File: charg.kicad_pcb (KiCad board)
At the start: 2 copper layers, 13 parts, among them IC1 SI3483DDV-T1-BE3, IC2 BQ25302RTER, J1 Screw_Terminal_01x04, J2 Screw_Terminal_01x04, J4 EN

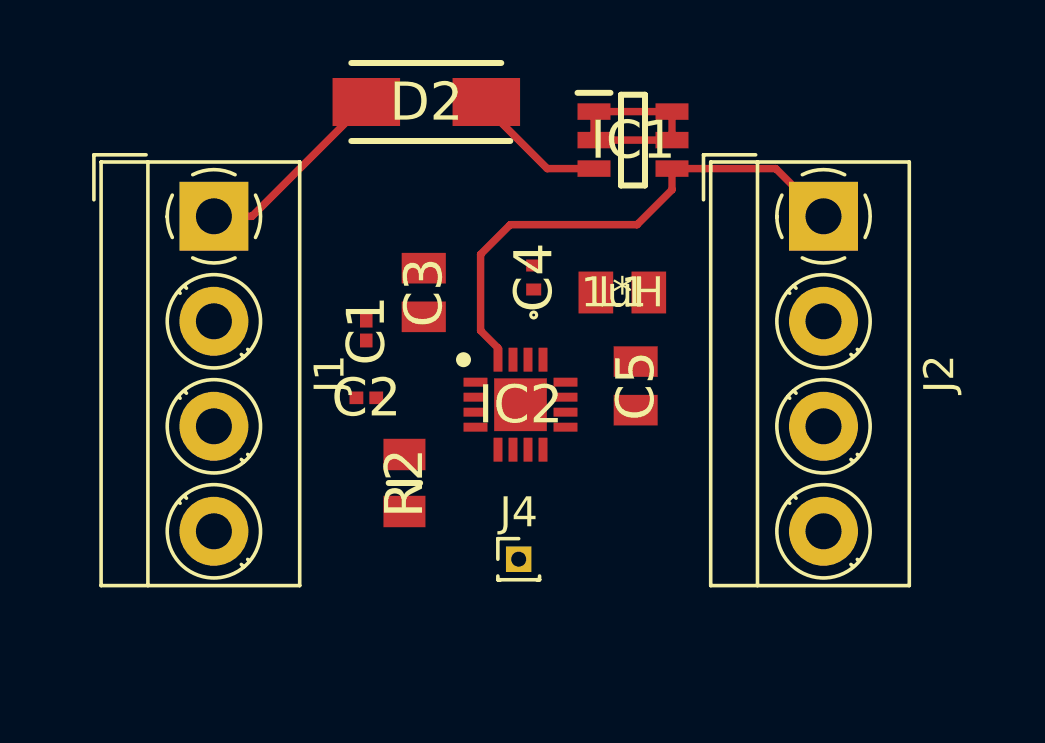
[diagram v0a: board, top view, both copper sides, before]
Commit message: PCB v1
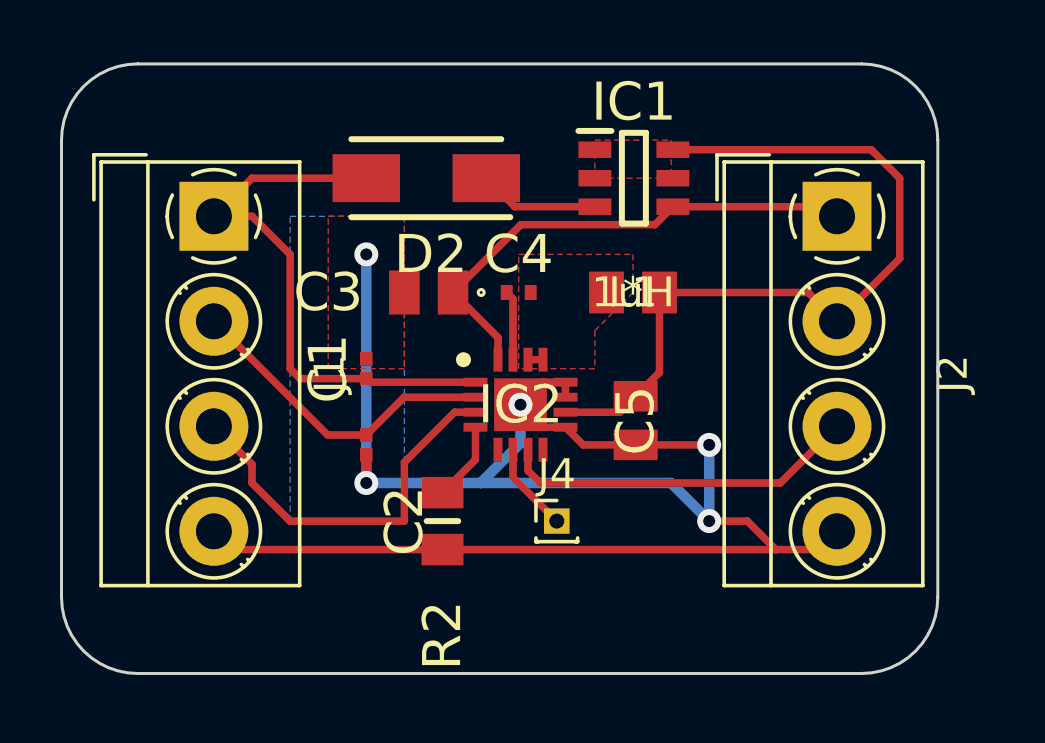
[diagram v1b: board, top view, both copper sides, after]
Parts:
- moved D2 2.54 mm to (145.5, 53.3)
- moved J4 1.80 mm to (149.9, 64.8)
- moved R2 1.80 mm to (146.1, 64.8)
- moved C2 1.57 mm to (143.5, 62.2), turned to -90 degrees
- moved IC1 1.27 mm to (152.4, 53.3)
- moved C1 1.27 mm to (143.5, 59.7)
- moved C5 1.16 mm to (152.5, 61.4)
- moved C4 0.71 mm to (148.6, 57.1), turned to 0 degrees
- moved J2 0.45 mm to (159.2, 54.6)
- moved L1 0.36 mm to (152.4, 57.1)
- moved C3 0.16 mm to (145.6, 57.1), turned to 180 degrees
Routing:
- net Earth: track 0.00 -> 59.3 mm, vias 0 -> 5
- net Net-(C5-Pad1): track 7.05 -> 26.3 mm
- net Net-(IC2-Pad3): track 0.00 -> 13.0 mm
- net Net-(C1-Pad1): track 6.66 -> 18.8 mm
- net Net-(IC2-Pad7): track 0.00 -> 12.0 mm
- net Net-(C2-Pad1): track 0.00 -> 10.8 mm
- net Net-(IC2-Pad6): track 0.00 -> 2.98 mm
- net Net-(IC2-Pad4): track 0.00 -> 2.64 mm
- net Net-(C4-Pad1): track 0.00 -> 2.33 mm
- net Net-(D2-Pad1): track 4.62 -> 4.01 mm
- net Net-(C4-Pad2): track 0.00 -> 0.50 mm
- added copper zone on B.Cu, net Earth
- added copper zone on F.Cu, net Earth
- added copper zone on F.Cu, net Net-(C4-Pad2)
- added copper zone on F.Cu, net Net-(C5-Pad1)
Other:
- board outline added: 29.2 x 20.3 mm
